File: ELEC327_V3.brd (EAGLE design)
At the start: 53 x 50 mm, 39 parts, among them J1 MJ-3502, U1 ADA4098-1HUJZ-RL7UJ-6_ADI-M, U2 ADA4098-1HUJZ-RL7UJ-6_ADI-M, U3 ADA4098-1HUJZ-RL7UJ-6_ADI-M, U4 LM833N/NOPB, U5 MAX619CPA+

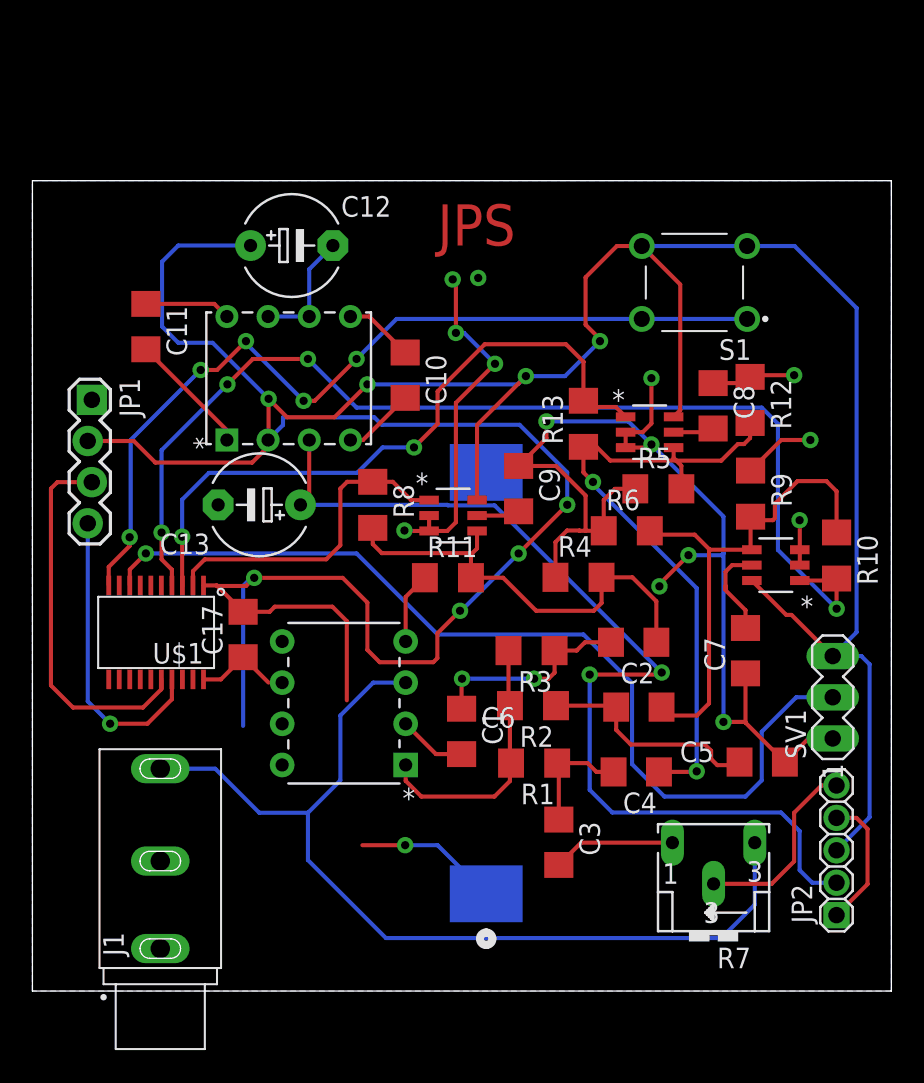
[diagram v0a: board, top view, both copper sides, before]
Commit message: Update ELEC327_V3.brd
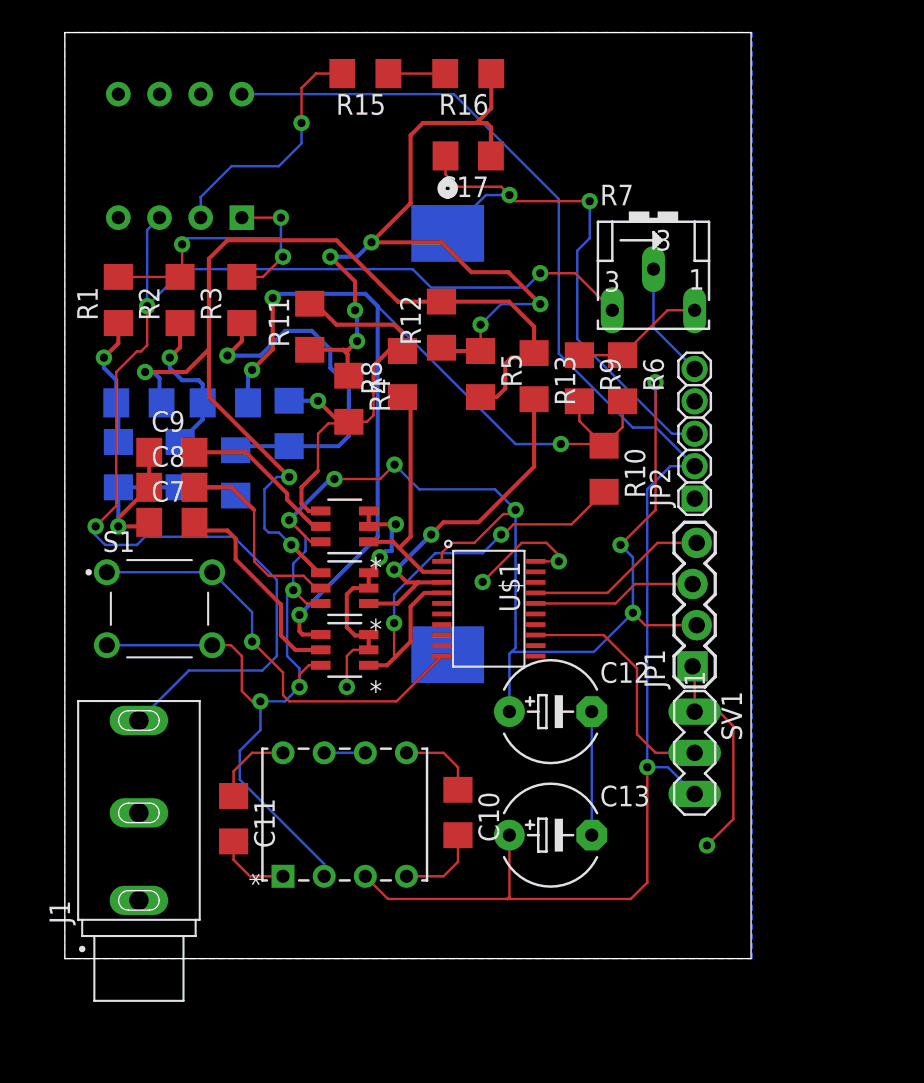
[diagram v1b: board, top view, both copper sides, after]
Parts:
- added R15, R16: (no value), rcl:R1206
- moved JP1 40.8 mm to (38.9, 18.0), turned to 90 degrees
- moved C5 40.3 mm to (7.11, 30.5), flipped to the bottom, turned to 270 degrees
- moved S1 38.7 mm to (5.84, 21.6), turned to 0 degrees
- moved R1 38.4 mm to (3.30, 40.6), turned to 90 degrees
- moved C4 38.2 mm to (4.57, 34.3), flipped to the bottom, turned to 0 degrees
- moved R7 36.8 mm to (36.3, 41.9), turned to 0 degrees
- moved C7 36.3 mm to (6.60, 26.9), turned to 0 degrees
- moved C3 35.8 mm to (3.30, 30.5), flipped to the bottom
- moved U4 35.3 mm to (10.9, 45.7), flipped to the bottom, turned to 90 degrees
- moved C8 33.8 mm to (6.60, 29.1), turned to 0 degrees
- moved R2 33.2 mm to (7.11, 40.6), turned to 90 degrees
- moved C12 32.9 mm to (30.0, 15.2)
- moved C17 32.6 mm to (24.9, 49.5), turned to 180 degrees
- moved C6 31.7 mm to (9.91, 34.3), flipped to the bottom, turned to 0 degrees
- moved C11 30.8 mm to (10.4, 8.64)
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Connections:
- new net N$14: R15.1, R16.2
- new net V-: R15.2, U4.2
- net 5V: now also SV1.3
- net DATA: now also U$1.13; no longer U$1.8
- net GND: now also R16.1; no longer U4.2
- net VCC: no longer SV1.3
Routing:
- net VCC: track 230.7 -> 146.4 mm, vias 9 -> 12
- net DATA: track 58.2 -> 15.2 mm, vias 1 -> 0
- net A3: track 67.7 -> 27.2 mm, vias 4 -> 2
- net 5V: track 61.4 -> 96.8 mm, vias 2 -> 1
- net N$7: track 31.5 -> 61.6 mm, vias 0 -> 4
- net BUTTON1: track 53.8 -> 27.0 mm, vias 5 -> 1
- net LEFT: track 59.1 -> 80.5 mm, vias 0 -> 3
- net N$5: track 40.2 -> 61.2 mm, vias 2 -> 3
- net A2: track 41.1 -> 22.3 mm
- net V-: track 0.00 -> 15.2 mm, vias 0 -> 1
- net GND: track 141.3 -> 127.4 mm
- net RST: track 23.3 -> 10.2 mm
- net N$2: track 12.8 -> 23.0 mm, vias 2 -> 1
- net N$8: track 2.53 -> 12.2 mm
- net TEST: track 18.6 -> 11.2 mm, vias 1 -> 0
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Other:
- board size 53 x 50 mm -> 42.3 x 57.1 mm
- board text removed: "JPS"
